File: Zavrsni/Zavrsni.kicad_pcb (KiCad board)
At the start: 2 copper layers, 103.4 x 61.2 mm, 21 parts, among them J1 12V Source, J3 Output A, J5 Conn_01x04, J6 Conn_02x19_Odd_Even, J7 Conn_02x19_Odd_Even, J8 Conn_01x06, U1 LM78M05_TO220, U2 L298N

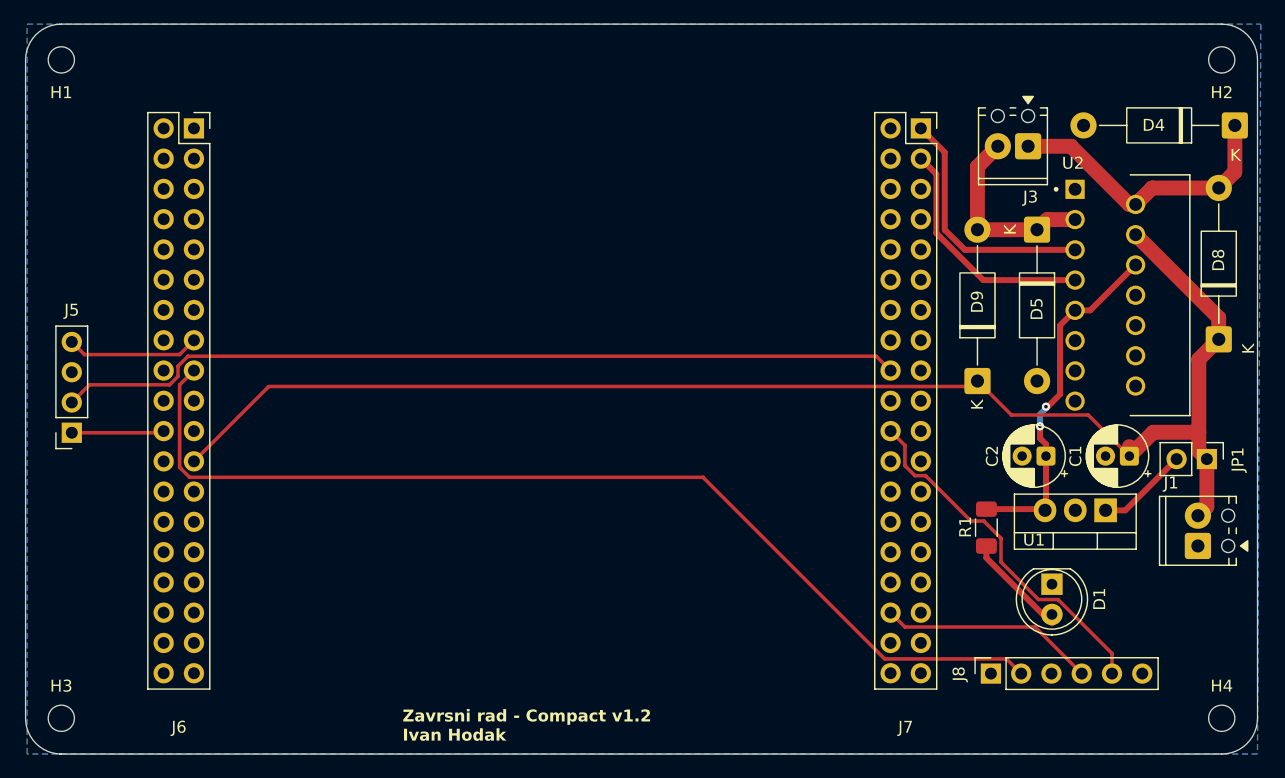
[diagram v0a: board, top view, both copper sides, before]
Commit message: New
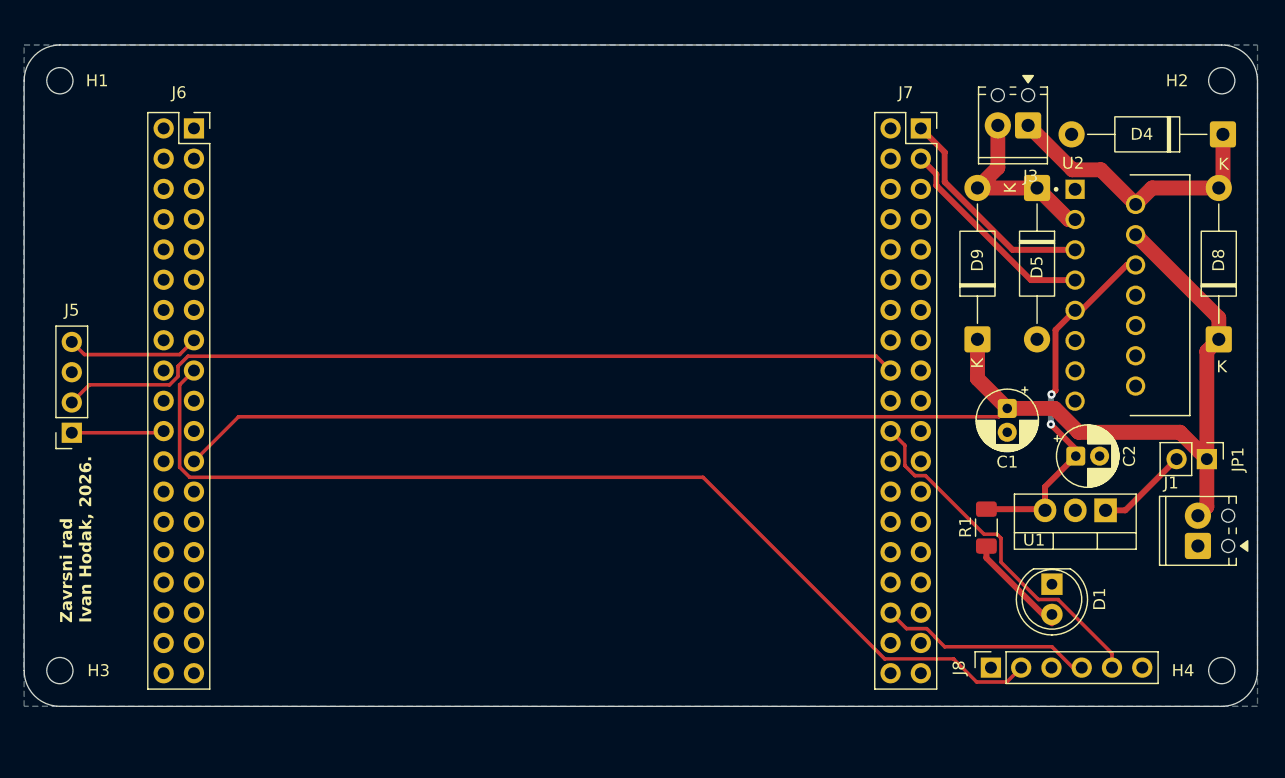
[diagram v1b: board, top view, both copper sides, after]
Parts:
- moved C1 11.0 mm to (193.2, 108.5), turned to -90 degrees
- moved H3 4.00 mm to (113.8, 130.5)
- moved H4 4.00 mm to (211.2, 130.5)
- moved D5 3.50 mm to (195.8, 90.0)
- moved D9 3.50 mm to (190.8, 102.7)
- moved C2 2.50 mm to (199.0, 112.5), turned to 0 degrees
- moved H1 1.75 mm to (113.8, 81.0)
- moved H2 1.75 mm to (211.2, 81.0)
- moved J3 1.75 mm to (195.0, 84.8)
- moved D4 1.25 mm to (211.3, 85.5)
- moved J8 0.50 mm to (191.9, 130.2)
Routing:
- net 12V: track 119.1 -> 122.6 mm
- net IN2: track 20.1 -> 17.7 mm
- net IN1: track 21.0 -> 18.6 mm
- net Vss: track 30.2 -> 31.4 mm
- net OUT2: track 16.3 -> 15.2 mm
- net 5V: track 86.4 -> 87.2 mm
- net RX: track 30.2 -> 29.7 mm
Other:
- board size 103.4 x 61.2 mm -> 103.5 x 55.5 mm
- board text added: "Zavrsni rad Ivan Hodak, 2026."
- board text removed: "Zavrsni rad - Compact v1.2 Ivan Hodak"

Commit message: New 3
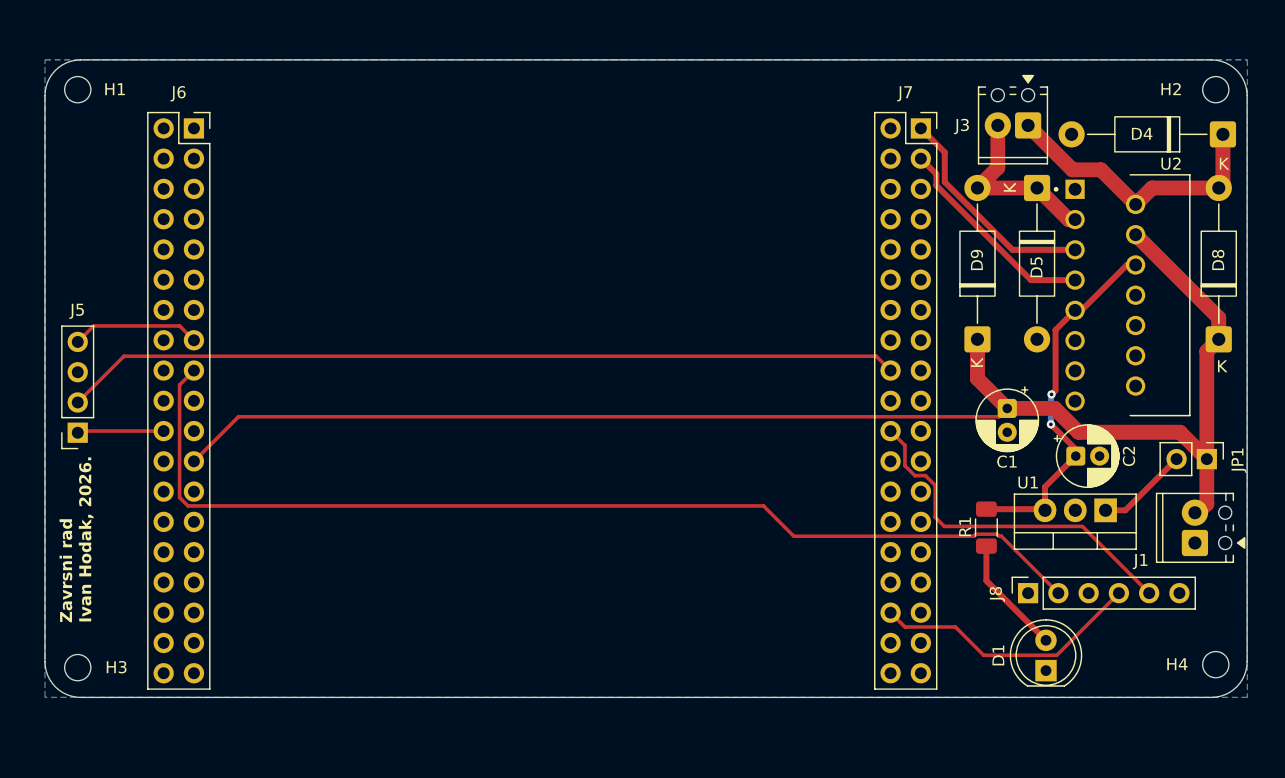
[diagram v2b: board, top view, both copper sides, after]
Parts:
- moved D1 7.27 mm to (196.5, 130.5), turned to 90 degrees
- moved J8 6.99 mm to (195.0, 124.0)
- moved H1 1.68 mm to (115.2, 81.8)
- moved H3 1.52 mm to (115.2, 130.2)
- moved H2 0.90 mm to (210.8, 81.8)
- moved H4 0.71 mm to (210.8, 130.0)
- moved J5 0.50 mm to (115.2, 110.5)
- moved J1 0.35 mm to (209.0, 119.8)
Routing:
- net TX: track 18.0 -> 22.8 mm
- net Net-(D1-A): track 8.77 -> 9.98 mm
- net 5V: track 87.2 -> 88.4 mm
- net SCL: track 71.3 -> 70.3 mm
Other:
- board size 103.5 x 55.5 mm -> 100.9 x 53.5 mm

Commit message: New 4
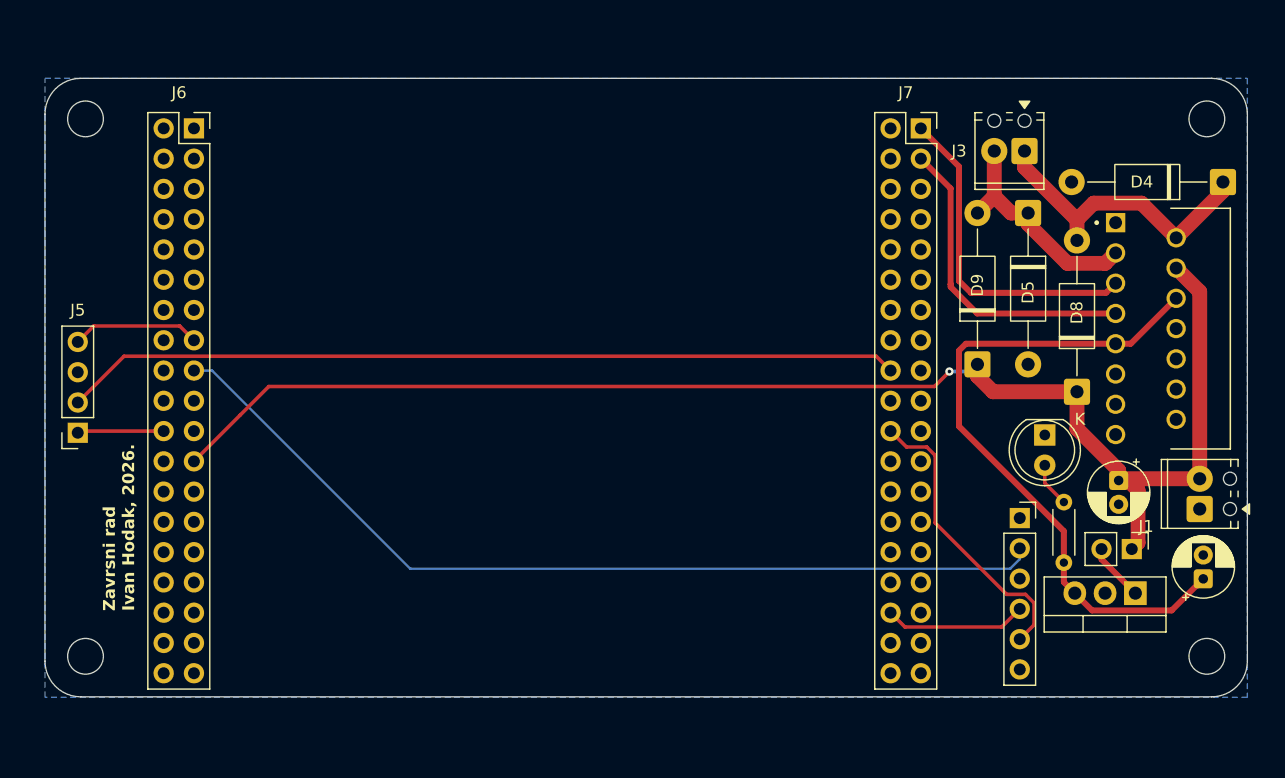
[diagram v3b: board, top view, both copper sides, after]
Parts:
- H1, H2, H3, H4: footprint MountingHole:MountingHole_2.2mm_M2_ISO7380 -> MountingHole:MountingHole_3mm
- R1: footprint Resistor_SMD:R_1206_3216Metric_Pad1.30x1.75mm_HandSolder -> Resistor_THT:R_Axial_DIN0204_L3.6mm_D1.6mm_P5.08mm_Horizontal
- moved D1 19.8 mm to (196.4, 110.7), turned to -90 degrees
- moved C2 14.9 mm to (209.7, 122.8), turned to 90 degrees
- moved D8 12.7 mm to (199.1, 107.1)
- moved C1 11.1 mm to (202.6, 114.5)
- moved JP1 9.83 mm to (203.7, 120.3)
- moved U1 7.39 mm to (204.0, 124.0)
- moved R1 7.13 mm to (198.0, 121.4), turned to 90 degrees
- moved J8 6.34 mm to (194.3, 117.7), turned to 0 degrees
- moved U2 4.40 mm to (202.3, 92.9)
- moved D4 4.00 mm to (211.3, 89.5)
- moved J1 2.88 mm to (209.4, 116.9)
- moved H2 2.56 mm to (210.0, 84.2)
- moved H1 2.53 mm to (115.9, 84.2)
- moved D5 2.23 mm to (195.0, 92.1)
- moved J3 2.17 mm to (194.7, 86.9)
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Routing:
- net Vss: track 31.4 -> 56.9 mm, vias 2 -> 0
- net 5V: track 88.4 -> 77.4 mm
- net TX: track 22.8 -> 12.0 mm
- net IN1: track 18.6 -> 28.0 mm
- net IN2: track 17.7 -> 26.6 mm
- net Net-(D1-A): track 9.98 -> 3.76 mm
- net RX: track 29.9 -> 24.9 mm
- net OUT2: track 15.2 -> 19.2 mm
- net Net-(JP1-B): track 7.74 -> 4.88 mm
- net 12V: track 122.7 -> 120.5 mm, vias 0 -> 1
- net OUT1: track 24.0 -> 25.7 mm
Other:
- board size 100.9 x 53.5 mm -> 100.9 x 51.9 mm
